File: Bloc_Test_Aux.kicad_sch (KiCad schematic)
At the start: 44 parts, among them Q29 2N7000, Q30 2N7000, Q31 2N7000, Q32 2N7000, Q33 2N7000, Q34 2N7000

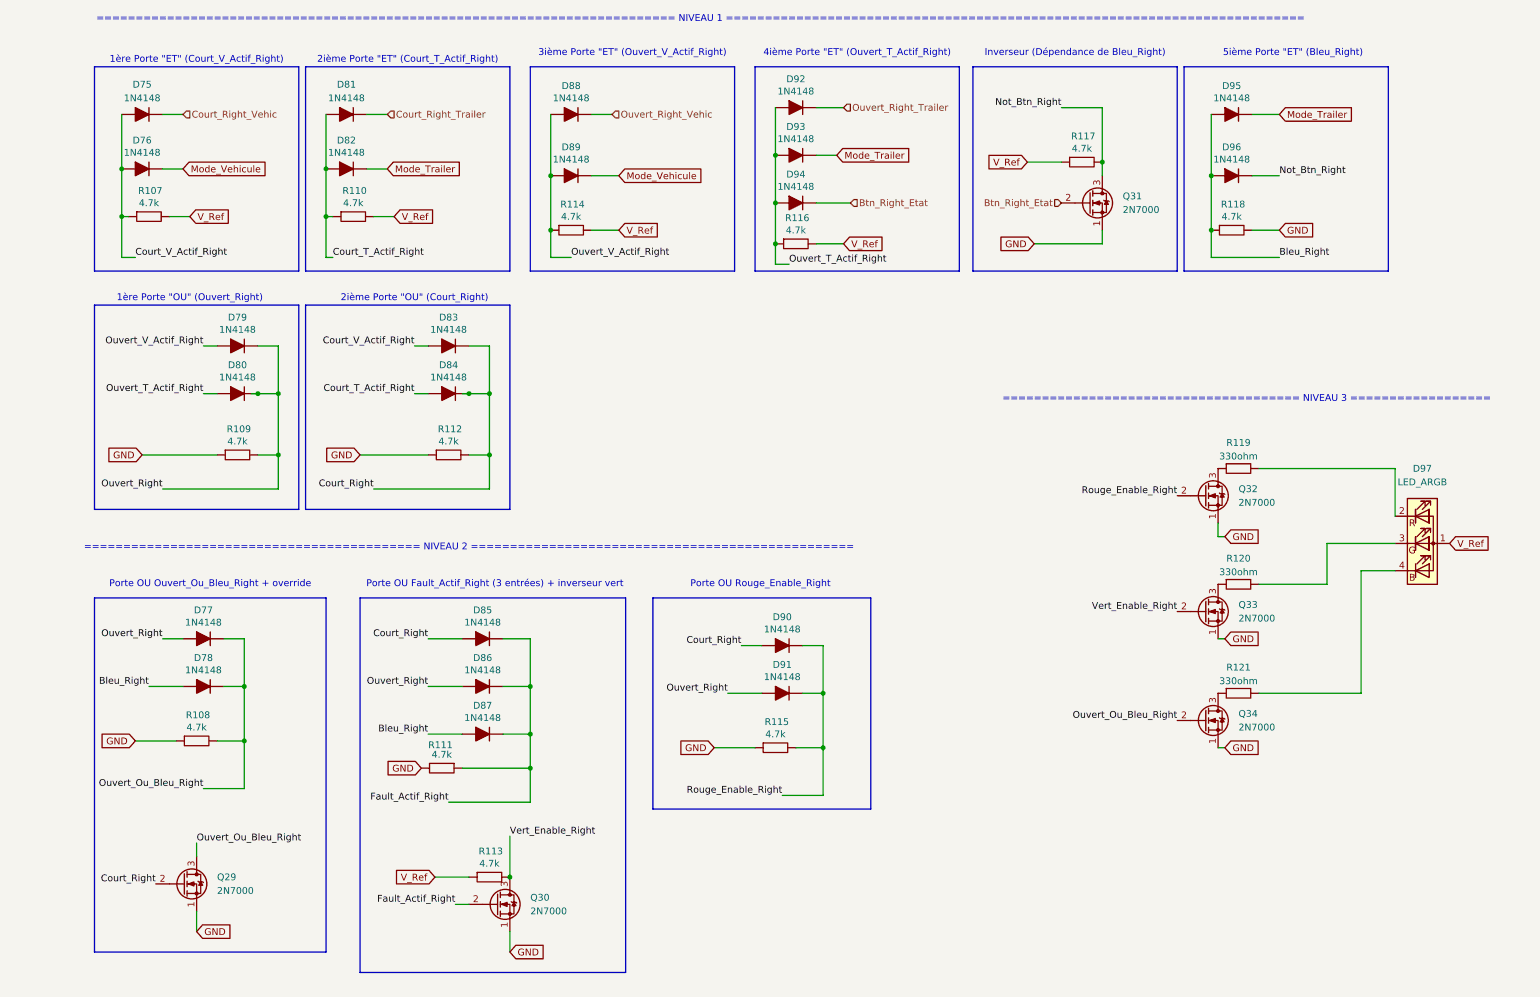
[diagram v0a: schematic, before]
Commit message: Add files via upload
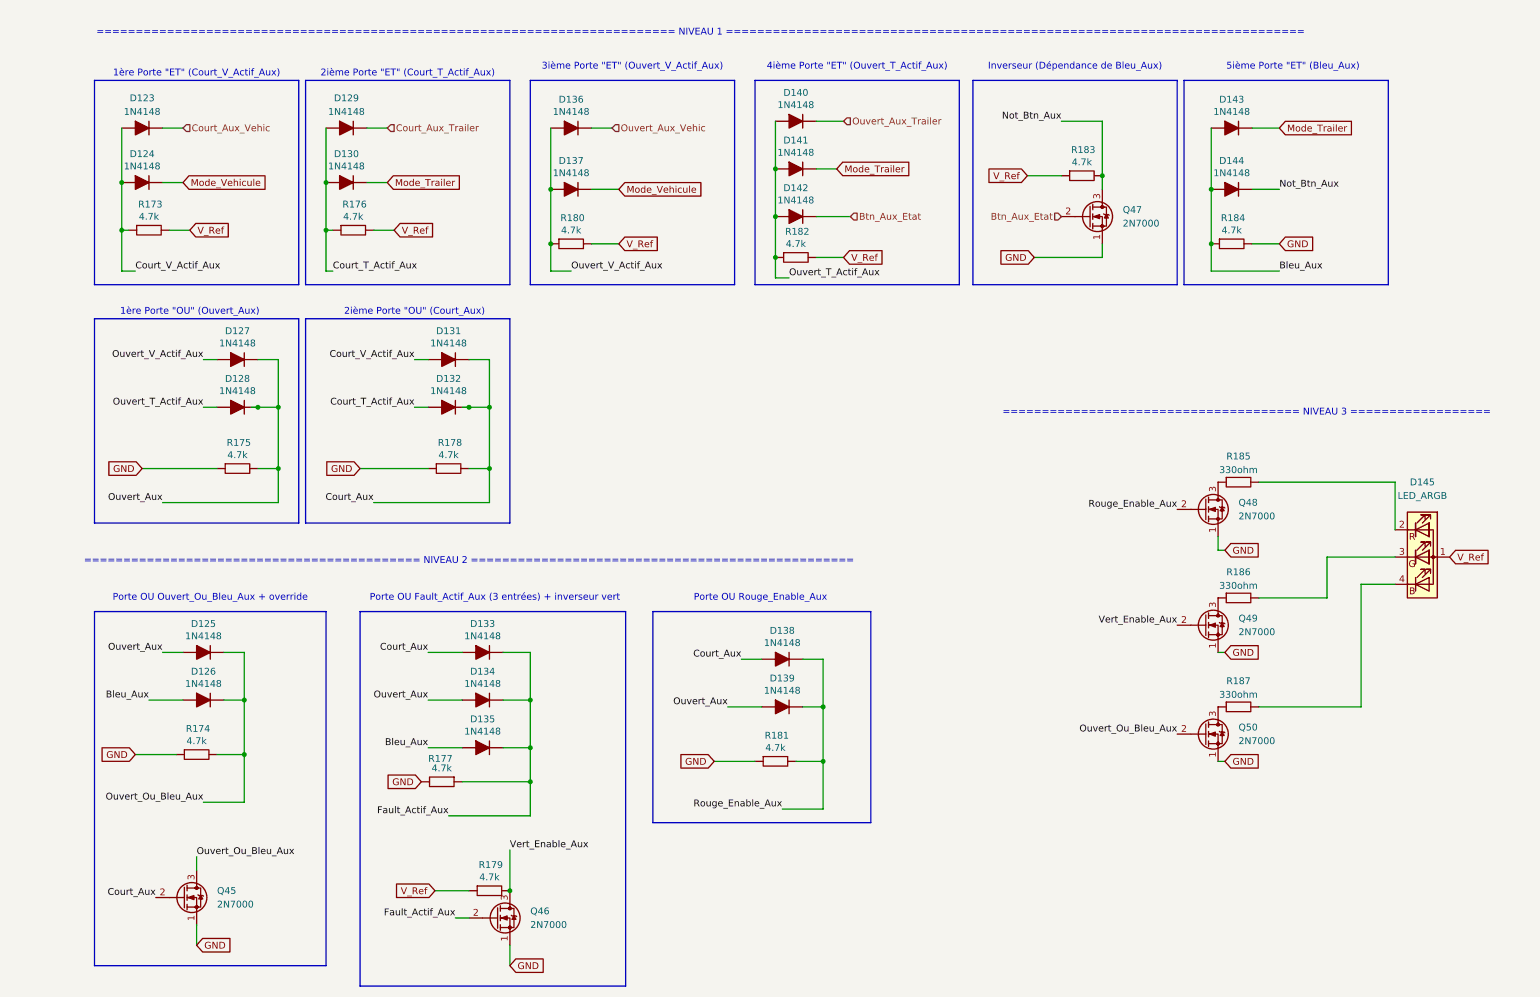
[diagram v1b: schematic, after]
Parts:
- removed D75, D76, D77, D78, D79, D80, D81, D82, D83, D84, D85, D86, D87, D88, D89, D90, D91, D92, D93, D94, D95, D96: 1N4148, PCM_Diode_THT_AKL:D_DO-35_SOD27_P7.62mm_Horizontal, symbol PCM_Diode_AKL:1N4148
- removed D97: LED_ARGB, symbol Device:LED_ARGB
- removed Q29, Q30, Q31, Q32, Q33, Q34: 2N7000, Package_TO_SOT_THT:TO-92_Inline, symbol Transistor_FET:2N7000
- removed R107, R108, R109, R110, R111, R112, R113, R114, R115, R116, R117, R118: 4.7k, Resistor_THT:R_Axial_DIN0207_L6.3mm_D2.5mm_P10.16mm_Horizontal, symbol PCM_SL_Resistors:4.7k
- removed R119, R120, R121: 330ohm, Resistor_THT:R_Axial_DIN0207_L6.3mm_D2.5mm_P10.16mm_Horizontal, symbol PCM_SL_Resistors:330ohm
- added D123, D124, D125, D126, D127, D128, D129, D130, D131, D132, D133, D134, D135, D136, D137, D138, D139, D140, D141, D142, D143, D144: 1N4148, PCM_Diode_THT_AKL:D_DO-35_SOD27_P7.62mm_Horizontal, symbol PCM_Diode_AKL:1N4148
- added D145: LED_ARGB, symbol Device:LED_ARGB
- added Q45, Q46, Q47, Q48, Q49, Q50: 2N7000, Package_TO_SOT_THT:TO-92_Inline, symbol Transistor_FET:2N7000
- added R173, R174, R175, R176, R177, R178, R179, R180, R181, R182, R183, R184: 4.7k, Resistor_THT:R_Axial_DIN0207_L6.3mm_D2.5mm_P10.16mm_Horizontal, symbol PCM_SL_Resistors:4.7k
- added R185, R186, R187: 330ohm, Resistor_THT:R_Axial_DIN0207_L6.3mm_D2.5mm_P10.16mm_Horizontal, symbol PCM_SL_Resistors:330ohm
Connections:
- net GND: now also Q45.1 (S), Q46.1 (S), Q47.1 (S), Q48.1 (S), Q49.1 (S), Q50.1 (S), R174.1, R175.1, R177.2, R178.1, R181.1, R184.2
- net Mode_Trailer: now also D130.1 (K), D141.1 (K), D143.1 (K)
- net Mode_Vehicule: now also D124.1 (K), D137.1 (K)
- net V_Ref: now also D145.1 (A), R173.2, R176.2, R179.1, R180.2, R182.2, R183.1
- new net: Q49.3 (D), R186.1
- new net: D145.3 (GK), R186.2
- new net: Q48.3 (D), R185.1
- new net: D145.2 (RK), R185.2
- new net: D145.4 (BK), R187.2
- new net: Q50.3 (D), R187.1
- new net Bleu_Aux: D126.2 (A), D135.2 (A), D143.2 (A), D144.2 (A), R184.1
- new net Btn_Aux_Etat: D142.1 (K), Q47.2 (G)
- new net Court_Aux: D131.1 (K), D132.1 (K), D133.2 (A), D138.2 (A), Q45.2 (G), R178.2
- new net Court_Aux_Trailer: D129.1 (K)
- new net Court_Aux_Vehic: D123.1 (K)
- new net Court_T_Actif_Aux: D129.2 (A), D130.2 (A), D132.2 (A), R176.1
- new net Court_V_Actif_Aux: D123.2 (A), D124.2 (A), D131.2 (A), R173.1
- new net Fault_Actif_Aux: D133.1 (K), D134.1 (K), D135.1 (K), Q46.2 (G), R177.1
- new net Not_Btn_Aux: D144.1 (K), Q47.3 (D), R183.2
- new net Ouvert_Aux: D125.2 (A), D127.1 (K), D128.1 (K), D134.2 (A), D139.2 (A), R175.2
- new net Ouvert_Aux_Trailer: D140.1 (K)
- new net Ouvert_Aux_Vehic: D136.1 (K)
- new net Ouvert_Ou_Bleu_Aux: D125.1 (K), D126.1 (K), Q45.3 (D), Q50.2 (G), R174.2
- new net Ouvert_T_Actif_Aux: D128.2 (A), D140.2 (A), D141.2 (A), D142.2 (A), R182.1
- new net Ouvert_V_Actif_Aux: D127.2 (A), D136.2 (A), D137.2 (A), R180.1
- new net Rouge_Enable_Aux: D138.1 (K), D139.1 (K), Q48.2 (G), R181.2
- new net Vert_Enable_Aux: Q46.3 (D), Q49.2 (G), R179.2
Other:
- note added: "1ère Porte "ET" (Court_V_Actif_Aux)"
- note added: "1ère Porte "OU" (Ouvert_Aux)"
- note added: "2ième Porte "ET" (Court_T_Actif_Aux)"
- note added: "2ième Porte "OU" (Court_Aux)"
- note added: "3ième Porte "ET" (Ouvert_V_Actif_Aux)"
- note added: "4ième Porte "ET" (Ouvert_T_Actif_Aux)"
- note added: "5ième Porte "ET" (Bleu_Aux)"
- note added: "Inverseur (Dépendance de Bleu_Aux)"
- note added: "Porte OU Fault_Actif_Aux (3 entrées) + inverseur vert"
- note added: "Porte OU Ouvert_Ou_Bleu_Aux + override"
- note added: "Porte OU Rouge_Enable_Aux"
- note removed: "1ère Porte "ET" (Court_V_Actif_Right)"
- note removed: "1ère Porte "OU" (Ouvert_Right)"
- note removed: "2ième Porte "ET" (Court_T_Actif_Right)"
- note removed: "2ième Porte "OU" (Court_Right)"
- note removed: "3ième Porte "ET" (Ouvert_V_Actif_Right)"
- note removed: "4ième Porte "ET" (Ouvert_T_Actif_Right)"
- note removed: "5ième Porte "ET" (Bleu_Right)"
- note removed: "Inverseur (Dépendance de Bleu_Right)"
- note removed: "Porte OU Fault_Actif_Right (3 entrées) + inverseur vert"
- note removed: "Porte OU Ouvert_Ou_Bleu_Right + override"
- note removed: "Porte OU Rouge_Enable_Right"

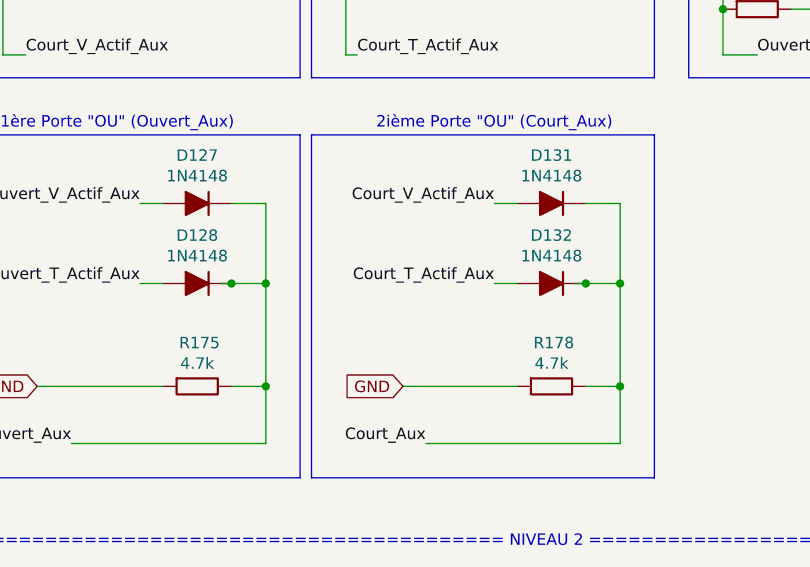
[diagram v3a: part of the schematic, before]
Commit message: Add files via upload
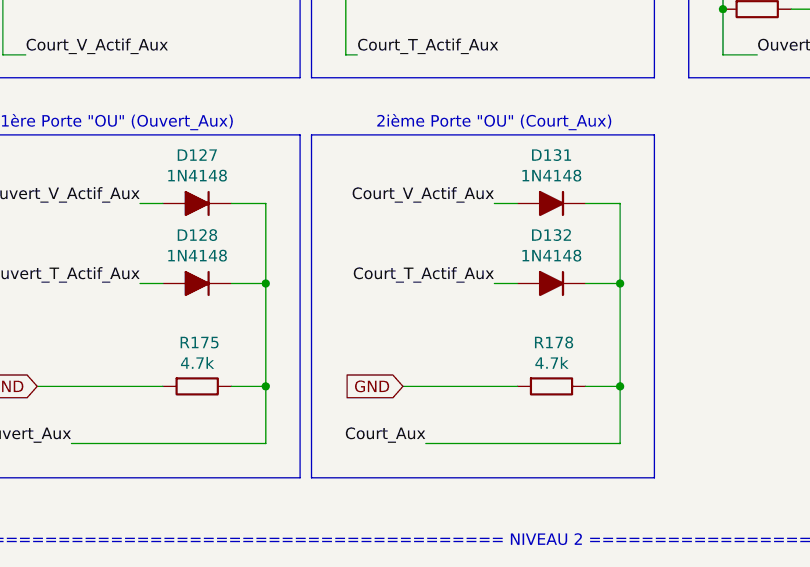
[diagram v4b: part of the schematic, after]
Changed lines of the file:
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@@
-	)
-	(junction
-		(at 91.44 88.9)
-		(diameter 0)
-		(color 0 0 0 0)
 	)
 	(junction
@@
 	)
 	(junction
-		(at 52.07 88.9)
-		(diameter 0)
-		(color 0 0 0 0)
-	)
-	(junction
 		(at 102.87 143.51)
 		(diameter 0)
@@
 	(wire
 		(pts
-			(xy 90.17 88.9) (xy 91.44 88.9)
-		)
-		(stroke
-			(width 0)
-			(type default)
-		)
-	)
-	(wire
-		(pts
 			(xy 26.67 46.99) (xy 26.67 55.88)
 		)
@@
 		)
 		(stroke
-			(width 0)
-			(type default)
-		)
-	)
-	(wire
-		(pts
-			(xy 50.8 88.9) (xy 52.07 88.9)
-		)
-		(stroke
